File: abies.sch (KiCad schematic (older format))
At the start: 3 parts

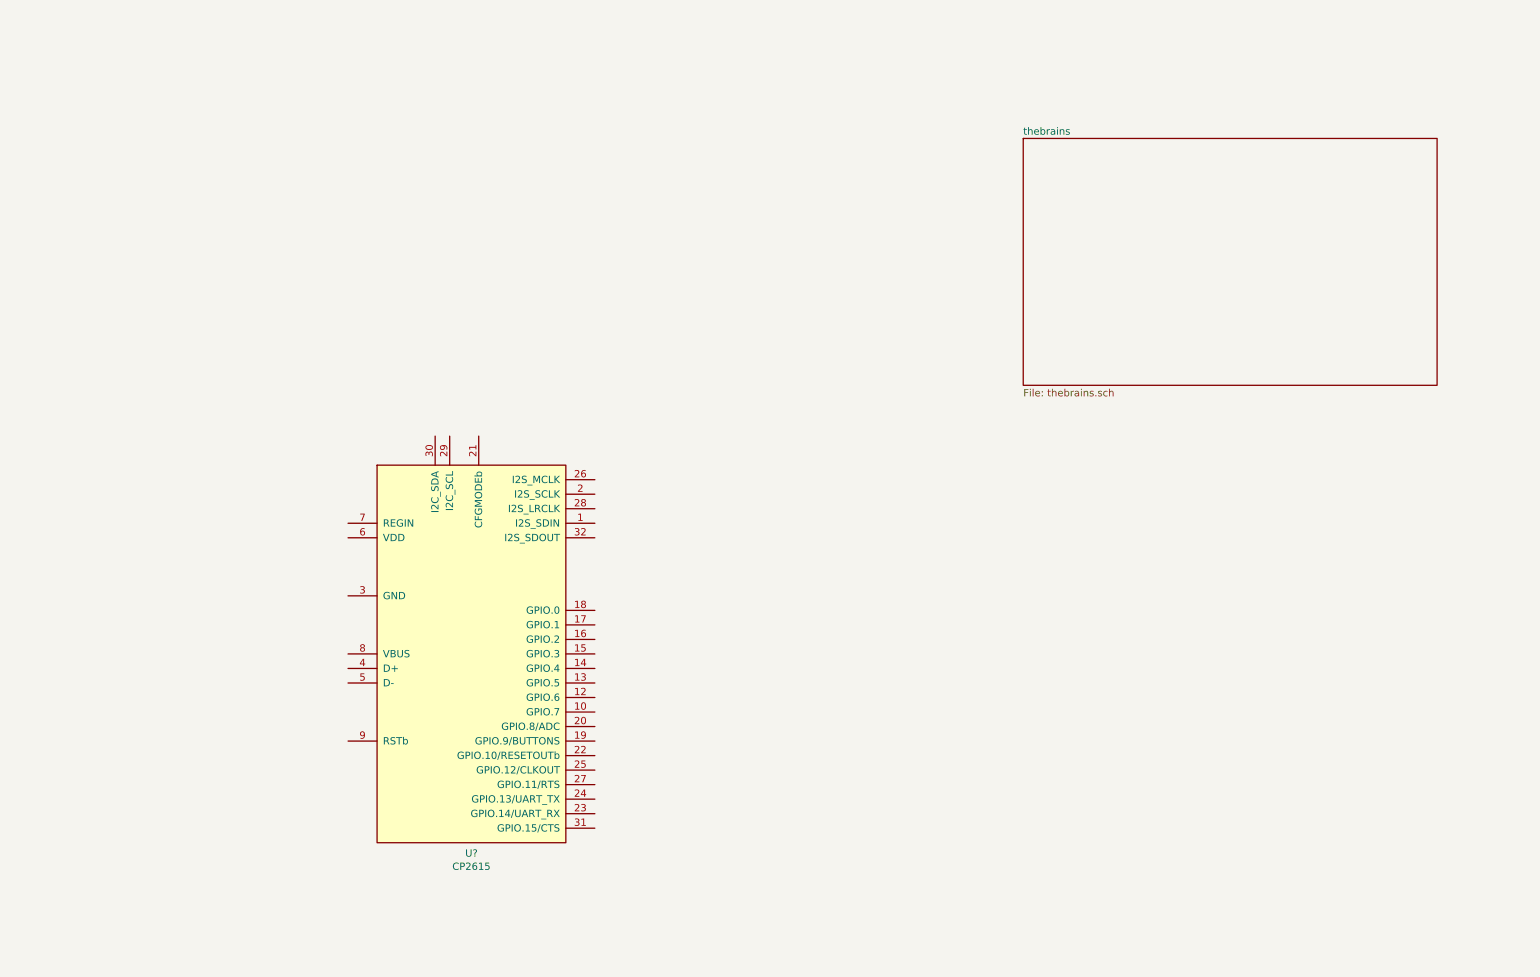
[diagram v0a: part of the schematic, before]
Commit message: More usb stuff
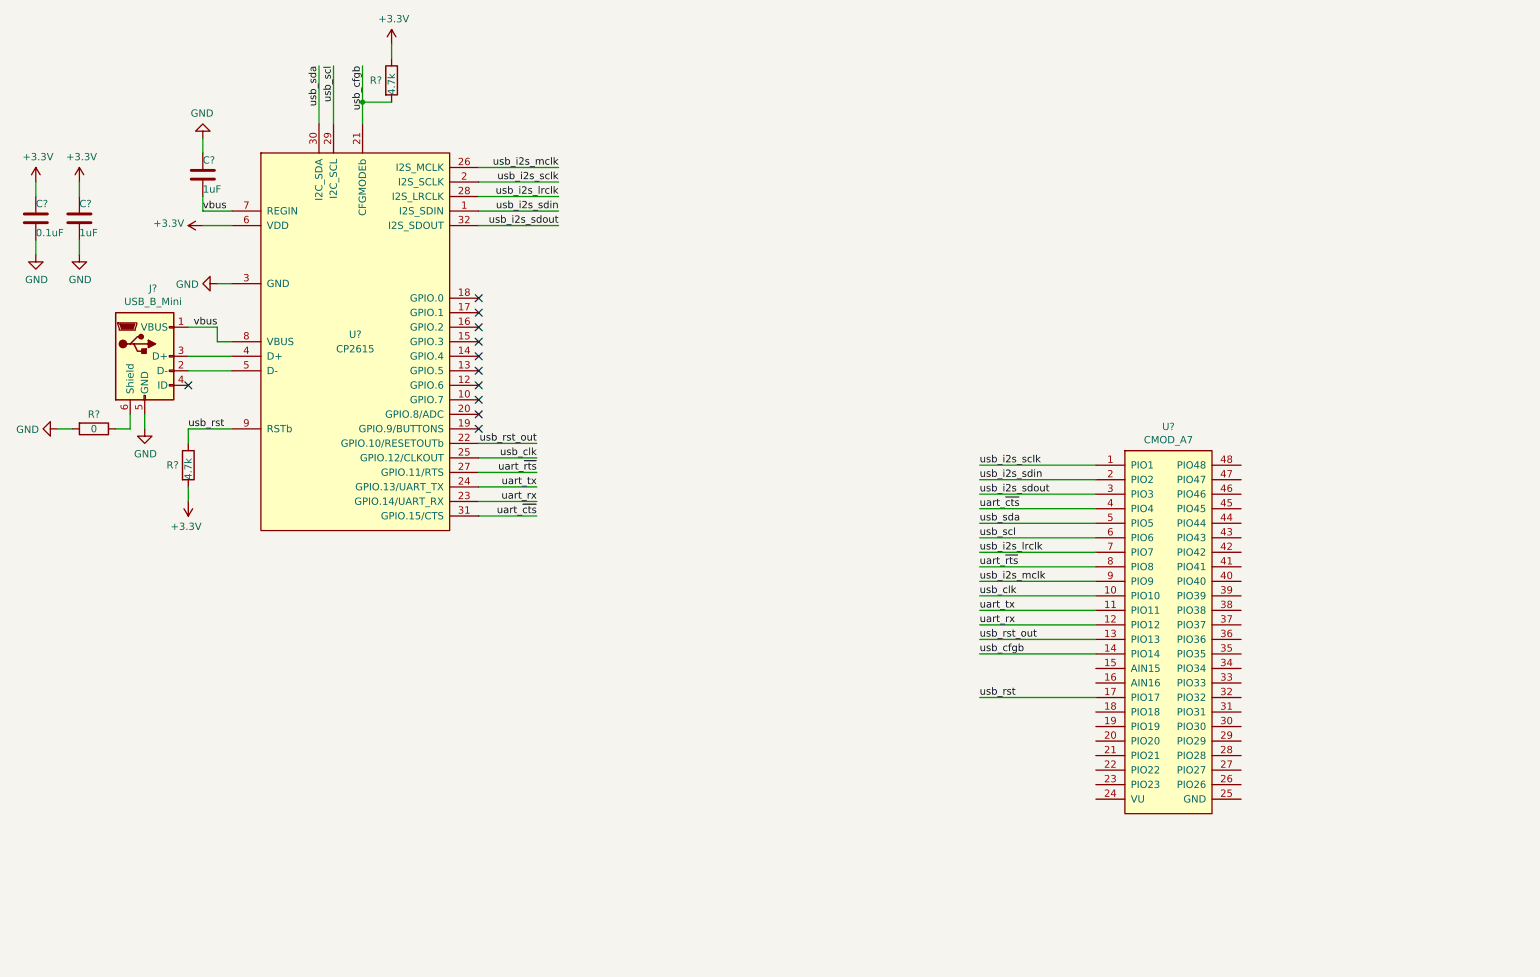
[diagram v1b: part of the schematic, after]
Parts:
- added C? (x2): 1uF, symbol Device:C
- added C?: 0.1uF, symbol Device:C
- added J?: USB_B_Mini, symbol Connector:USB_B_Mini
- added R?: 0, symbol Device:R
- added R? (x2): 4.7k, symbol Device:R
- added U?: CMOD_A7, symbol fpga_dev:CMOD_A7
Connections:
- net usb_i2s_sdin: now reaches U?.1 (I2S_SDIN)
- net usb_i2s_sdin: now also U?.2 (PIO2)
- net usb_i2s_sclk: now reaches U?.2 (I2S_SCLK)
- net usb_i2s_sclk: now also U?.1 (PIO1)
- net usb_cfgb: now reaches U?.21 (CFGMODEb)
- net usb_cfgb: now also R?.2, U?.14 (PIO14)
- net usb_rst_out: now reaches U?.22 (GPIO.10/RESETOUTb)
- net usb_rst_out: now also U?.13 (PIO13)
- net uart_rx: now reaches U?.23 (GPIO.14/UART_RX)
- net uart_rx: now also U?.12 (PIO12)
- net uart_tx: now reaches U?.24 (GPIO.13/UART_TX)
- net uart_tx: now also U?.11 (PIO11)
- net usb_clk: now reaches U?.25 (GPIO.12/CLKOUT)
- net usb_clk: now also U?.10 (PIO10)
- net usb_i2s_mclk: now reaches U?.26 (I2S_MCLK)
- net usb_i2s_mclk: now also U?.9 (PIO9)
- net uart_~rts~: now reaches U?.27 (GPIO.11/RTS)
- net uart_~rts~: now also U?.8 (PIO8)
- net usb_i2s_lrclk: now reaches U?.28 (I2S_LRCLK)
- net usb_i2s_lrclk: now also U?.7 (PIO7)
- net usb_scl: now reaches U?.29 (I2C_SCL)
- net usb_scl: now also U?.6 (PIO6)
- net GND: now reaches U?.3 (GND), U?.GND (33)
- net GND: now also C?.1, C?.2, C?.2, J?.5 (GND), R?.2
- net usb_sda: now reaches U?.30 (I2C_SDA)
- net usb_sda: now also U?.5 (PIO5)
- net uart_~cts~: now reaches U?.31 (GPIO.15/CTS)
- net uart_~cts~: now also U?.4 (PIO4)
- net usb_i2s_sdout: now reaches U?.32 (I2S_SDOUT)
- net usb_i2s_sdout: now also U?.3 (PIO3)
- net at U?.4 (D+): now also J?.3 (D+)
- net at U?.5 (D-): now also J?.2 (D-)
- net +3V3: now reaches U?.6 (VDD)
- net +3V3: now also C?.1, C?.1, R?.1, R?.2
- net vbus: now reaches U?.7 (REGIN)
- net vbus: now also U?.8 (VBUS), C?.2, J?.1 (VBUS)
- net usb_rst: now reaches U?.9 (RSTb)
- net usb_rst: now also R?.1, U?.17 (PIO17)
- new net: J?.6 (Shield), R?.1
- no-connect marks 0 -> 11
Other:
- moved on the sheet: U?

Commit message: more stuff
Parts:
- removed C? (x2): 1uF, symbol Device:C
- removed C?: 0.1uF, symbol Device:C
- removed J?: USB_B_Mini, symbol Connector:USB_B_Mini
- removed R?: 0, symbol Device:R
- removed R? (x2): 4.7k, symbol Device:R
- removed U?: CP2615, Package_DFN_QFN:QFN-32-1EP_5x5mm_P0.5mm_EP3.7x3.7mm_ThermalVias, symbol audio_digital:CP2615
- removed U?: CS4350, Package_SO:TSSOP-24_4.4x7.8mm_P0.65mm, symbol audio_digital:CS4350
- added C? (x2): 18pf, symbol Device:C
- added C?: 10uF, symbol Device:C
- added C? (x2): 3.3uF, symbol Device:CP
- added C? (x2): 10uF, symbol Device:CP
- added C? (x4): 0.1uF, symbol Device:C
- added C? (x3): 1uF, symbol Device:CP
- added F?: ~, symbol Device:Fuse
- added FB?: ~, symbol Device:Ferrite_Bead
- added J?: USB_B_Mini, symbol Connector:USB_B_Mini
- added R? (x2): 22, symbol Device:R
- added R? (x3): 10k, symbol Device:R
- added R? (x2): 470, symbol Device:R
- added U?: STM32F105RBTx, Package_QFP:LQFP-64_10x10mm_P0.5mm, symbol MCU_ST_STM32F1:STM32F105RBTx
- added U?: CS4344, Package_SO:TSSOP-10_3x3mm_P0.5mm, symbol audio_digital:CS4344
- added Y?: 8MHz, symbol Device:Crystal
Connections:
- net +3V3: now also U?.3 (VL), U?.6 (VD), R?.1, U?.13 (VDDA), U?.19 (VDD), U?.32 (VDD), U?.48 (VDD), U?.64 (VDD)
- net GND: now also U?.14 (GND), U?.25 (GND), U?.5 (GND), C?.1, C?.1, C?.1, C?.2, C?.2, C?.2, C?.2, C?.2, C?.2, C?.2, C?.2, C?.2, J?.5 (GND), R?.1, R?.2, U?.12 (VSSA), U?.18 (VSS), U?.31 (VSS), U?.47 (VSS), U?.63 (VSS), U?.8 (AGND)
- net adc_m0: now reaches U?.1 (M0)
- net adc_m0: now also U?.29 (PIO29)
- net at U?.11 (VQ): now also C?.1, C?.2
- net +3.3VA: now reaches U?.13 (VA)
- net +3.3VA: now also C?.1, C?.1, U?.9 (VA)
- net at U?.15 (FILT+): now also C?.1, C?.2
- net adc_m1: now reaches U?.16 (M1)
- net adc_m1: now also U?.30 (PIO30)
- net i2s_clk3: now reaches U?.2 (MCLK)
- net i2s_sd3: now reaches U?.4 (SDOUT)
- net i2s_sd3: now also U?.28 (PIO28), R?.2
- net i2s_sck3: now reaches U?.7 (SCLK)
- net i2s_sck3: now also U?.27 (PIO27)
- net i2s_lrck3: now reaches U?.8 (LRCK)
- net i2s_lrck3: now also U?.26 (PIO26)
- net adc_~rst~: now reaches U?.9 (~RST)
- net i2s_mck2: now reaches U?.45 (PIO45)
- net i2s_mck2: now also U?.4 (MCLK)
- net i2s_lrck2: now reaches U?.46 (PIO46)
- net i2s_lrck2: now also U?.3 (LRCK)
- net i2s_sck2: now reaches U?.47 (PIO47)
- net i2s_sck2: now also U?.2 (SCLK)
- net i2s_sd2: now reaches U?.48 (PIO48)
- net i2s_sd2: now also U?.1 (SDIN)
- net uart_rx: no longer names the net of U?.12 (PIO12)
- net uart_tx: no longer names the net of U?.11 (PIO11)
- net uart_~cts~: no longer names the net of U?.4 (PIO4)
- net uart_~rts~: no longer names the net of U?.8 (PIO8)
- net usb_cfgb: no longer names the net of U?.14 (PIO14)
- net usb_clk: no longer names the net of U?.10 (PIO10)
- net usb_i2s_lrclk: no longer names the net of U?.7 (PIO7)
- net usb_i2s_mclk: no longer names the net of U?.9 (PIO9)
- net usb_i2s_sclk: no longer names the net of U?.1 (PIO1)
- net usb_i2s_sdin: no longer names the net of U?.2 (PIO2)
- net usb_i2s_sdout: no longer names the net of U?.3 (PIO3)
- net usb_rst: no longer names the net of U?.17 (PIO17)
- net usb_rst_out: no longer names the net of U?.13 (PIO13)
- net usb_scl: no longer names the net of U?.6 (PIO6)
- net usb_sda: no longer names the net of U?.5 (PIO5)
- new net: F?.2, J?.1 (VBUS)
- new net: J?.2 (D-), R?.2
- new net: J?.3 (D+), R?.2
- new net: C?.1, U?.5 (PD0), Y?.1
- new net: C?.1, U?.6 (PD1), Y?.2
- new net: F?.1, FB?.2
- new net: C?.1, U?.10 (AOUTR)
- new net: C?.1, C?.1, U?.5 (VQ)
- new net: C?.1, U?.6 (FILT+)
- new net: C?.1, U?.7 (AOUTL)
- new net: C?.2, R?.1, R?.1
- new net: C?.2, R?.1, R?.2
- new net +5V: C?.2, FB?.1
- new net i2s_lrck0: U?.33 (PB12)
- new net i2s_lrck1: U?.50 (PA15)
- new net i2s_mck0: U?.37 (PC6)
- new net i2s_mck1: U?.38 (PC7)
- new net i2s_sck0: U?.34 (PB13)
- new net i2s_sck1: U?.55 (PB3)
- new net i2s_sd0: U?.36 (PB15)
- new net i2s_sd1: U?.57 (PB5)
- new net usb_d+: R?.1, U?.45 (PA12)
- new net usb_d-: R?.1, U?.44 (PA11)
- no-connect marks 11 -> 2
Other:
- note added: "Output Amplifier"
- note added: "Stereo DAC"
- note added: "USB"
- note added: "i2s0: USB to FPGA Bridge\ni2s1: FPGA to USB Bridge\ni2s2: FPGA to DAC\ni2s3: ADC to FPGA"
- moved on the sheet: U?
